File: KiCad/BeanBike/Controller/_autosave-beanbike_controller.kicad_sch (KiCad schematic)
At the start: 1 part, among them U1 ESP32-WROOM-32

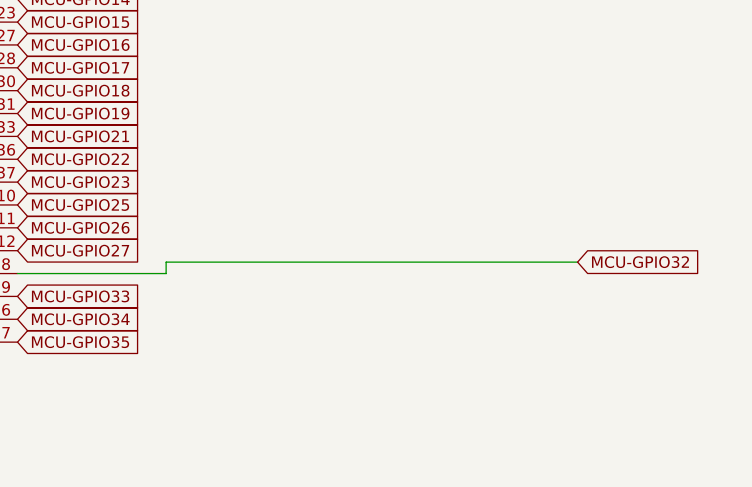
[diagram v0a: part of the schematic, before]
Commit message: Power Circuit V1
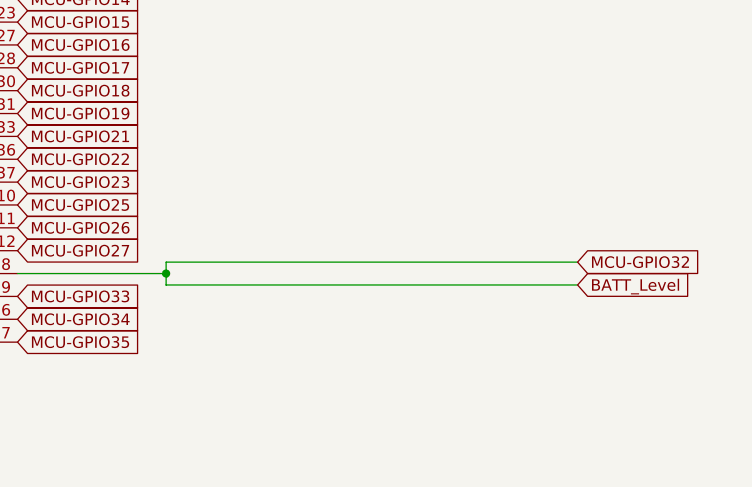
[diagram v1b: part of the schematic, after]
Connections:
- net MCU-GPIO32 renamed BATT_Level
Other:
- company: (none) -> Ginobeano
- title: (none) -> BeanBike Controller MCU
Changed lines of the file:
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@@
 	(generator_version "9.0")
 	(paper "A4")
+	(title_block
+		(title "BeanBike Controller MCU")
+		(date "2025-10-10")
+		(rev "1")
+		(company "Ginobeano")
+	)
+	(junction
+		(at 167.64 130.81)
+		(diameter 0)
+		(color 0 0 0 0)
+	)
 	(no_connect
 		(at 120.65 113.03)
@@
 	(wire
 		(pts
-			(xy 167.64 130.81) (xy 151.13 130.81)
+			(xy 167.64 130.81) (xy 167.64 132.08)
 		)
 		(stroke
@@
 	(wire
 		(pts
-			(xy 167.64 129.54) (xy 167.64 130.81)
+			(xy 167.64 130.81) (xy 151.13 130.81)
 		)
 		(stroke
@@
 		)
 	)
+	(wire
+		(pts
+			(xy 167.64 129.54) (xy 167.64 130.81)
+		)
+		(stroke
+			(width 0)
+			(type default)
+		)
+	)
+	(wire
+		(pts
+			(xy 167.64 132.08) (xy 213.36 132.08)
+		)
+		(stroke
+			(width 0)
+			(type default)
+		)
+	)
 	(global_label "MCU-GPIO34"
 		(shape input)
@@
 			(effects
 				(font
+					(size 1.27 1.27)
+				)
+				(justify left)
+				(hide yes)
+			)
+		)
+	)
+	(global_label "BATT_Level"
+		(shape input)
+		(at 213.36 132.08 0)
+		(fields_autoplaced yes)
+		(effects
+			(font
+				(size 1.27 1.27)
+			)
+			(justify left)
+		)
+		(property "Intersheetrefs" "${INTERSHEET_REFS}"
+			(at 226.4447 132.08 0)
+			(effects
+				(font
